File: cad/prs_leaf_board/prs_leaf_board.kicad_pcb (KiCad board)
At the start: 2 copper layers, 152.4 x 76.2 mm, 13 parts, among them J101 Conn_01x07

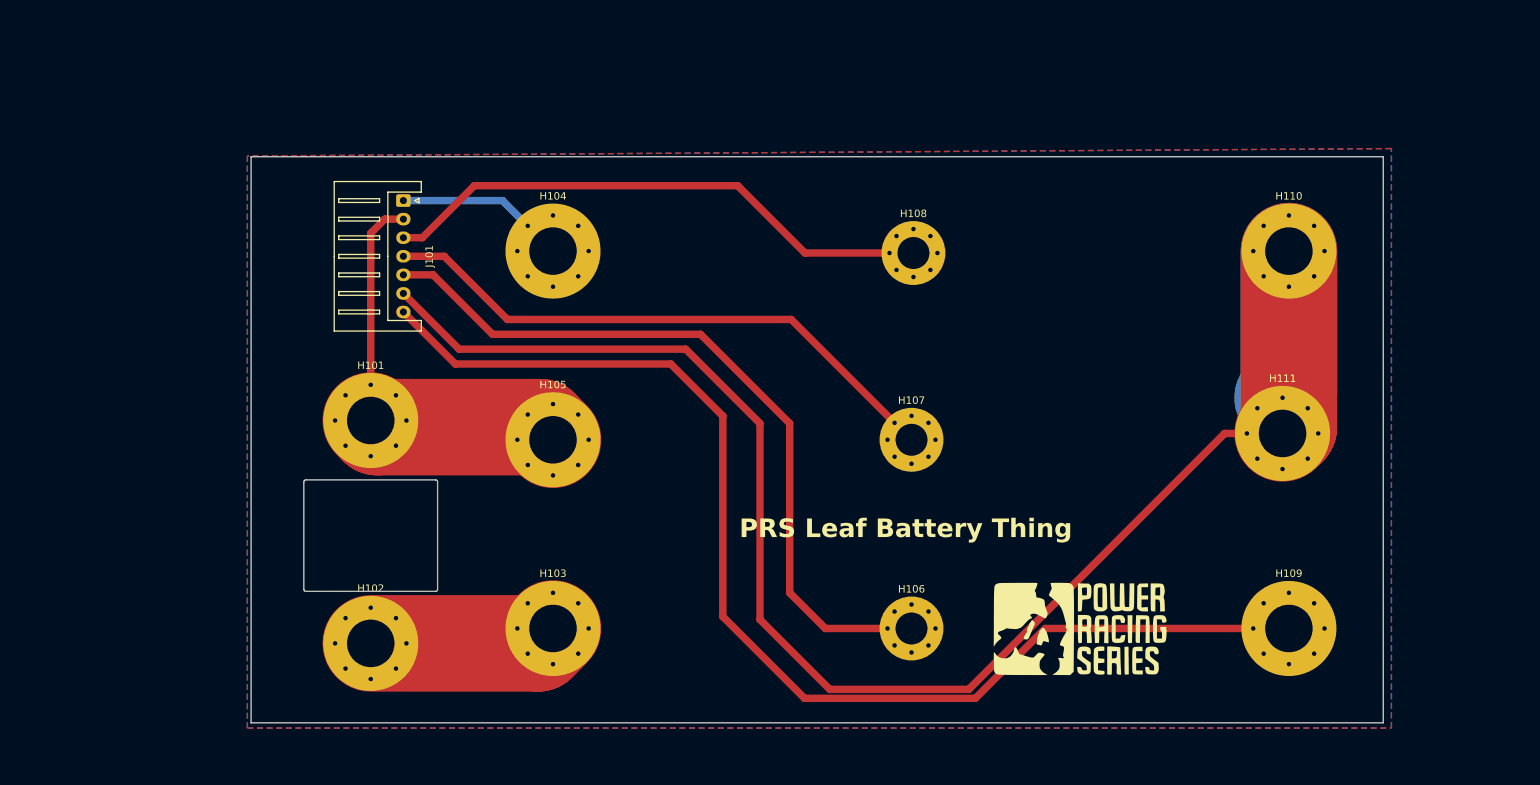
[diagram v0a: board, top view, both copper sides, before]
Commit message: rev2
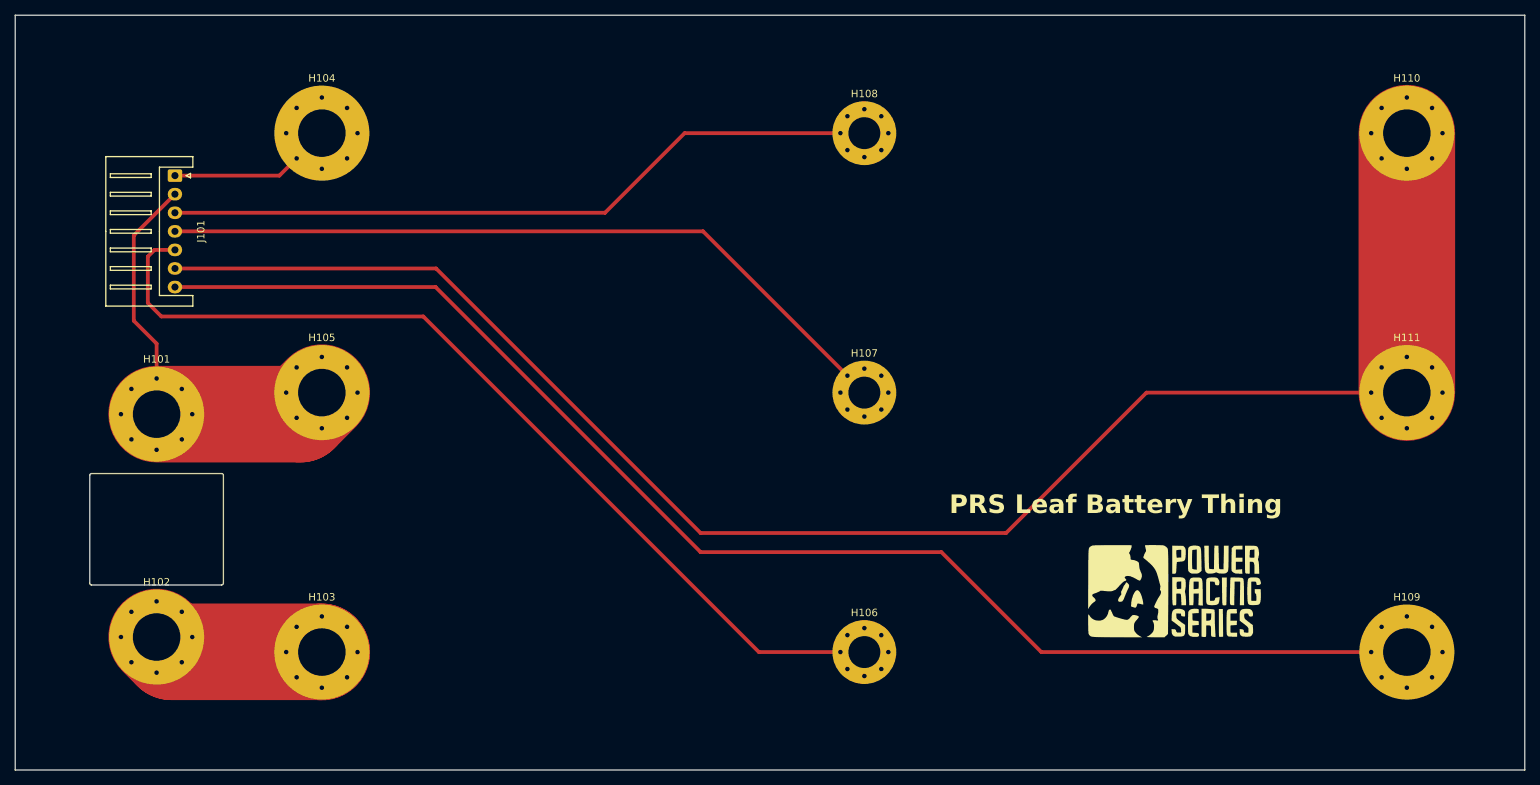
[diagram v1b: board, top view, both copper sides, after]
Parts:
- moved H104 34.9 mm to (73.0, 34.9)
- moved H105 31.8 mm to (73.0, 69.8)
- moved H103 31.3 mm to (73.0, 104.8)
- moved J101 30.9 mm to (53.2, 40.6)
- moved H101 28.8 mm to (50.8, 72.8)
- moved H102 28.8 mm to (50.8, 102.8)
- moved H110 22.5 mm to (219.1, 34.9)
- moved H111 17.6 mm to (219.1, 69.8)
- moved H108 17.4 mm to (146.1, 34.9)
- moved H109 16.2 mm to (219.1, 104.8)
- moved G*** 13.7 mm to (188.0, 96.5)
- moved H107 8.98 mm to (146.1, 69.8)
- moved H106 7.10 mm to (146.1, 104.8)
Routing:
- net Net-(J101-Pin_7): track 160.4 -> 186.2 mm
- net Net-(J101-Pin_5): track 101.5 -> 126.2 mm
- net Net-(J101-Pin_4): track 78.6 -> 101.8 mm
- net Net-(J101-Pin_3): track 75.3 -> 97.2 mm
- net Net-(J101-Pin_6): track 215.2 -> 223.3 mm
- net Net-(H102-Pad1): track 25.4 -> 23.1 mm
- net Net-(J101-Pin_1): track 23.0 -> 22.1 mm
- net Net-(J101-Pin_2): track 56.0 -> 56.6 mm
- removed copper zone on B.Cu, net (none)
- removed copper zone on F.Cu, net (none)
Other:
- board size 152.4 x 76.2 mm -> 203.2 x 101.6 mm
